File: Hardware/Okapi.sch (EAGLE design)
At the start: 247 parts, among them IC1 ATMEGA1284M, J1 CONN_82.54_SCREW, J3 CONN_42.54_SCREW, J4 CONN_82.54_SCREW, J9 B_SERIES_M.2EKEY_NOPROG, Q1 DMG3404, Q2 DMG3404, Q3 FDN360P, Q4 2N7002, Q5 FDN360P, Q6 DMG3404, Q7 2N7002, Q8 2N7002, U1 TLV61220DBV, U10 TPS22917DBV, U11 SN74AUP1G04YFP, U12 SN74AUP1G04YFP, U13 SN74AUP1G04YFP, U14 SN74AUP2G08DQE, U15 SN74AUP2G08DQE, U16 SN74AUP2G08DQE, U17 MIC2544MSOP, U18 MIC2544MSOP, U19 MIC2544MSOP, U2 TPS62822DLC, U20 MIC2544MSOP, U21 TPS22917DBV, U22 TPS22917DBV, U23 FT231X-Q, U24 SN74LVC1G3157DRL, U25 SN74AUP3G34DCU, U26 TXS0102DQM, U27 TXS0104RGY, U28 TCA9406DCU, U29 TXS0104RGY, U3 TPS61032RSA, U30 MCP4726A2SOT-23, U31 BME280, U32 PAC1934QFN, U33 ADS1115, U34 TXS0102DQM, U35 MB85RC, U36 TCA9406DCU, U37 TLV3691DCK, U38 MLX90393, U39 MIC94094C6, U40 SN74AHC1G86DCK, U41 MCP23018QFN, U42 TXS0104RGY, U43 BMA456, U44 VEML6030, U45 PCA9634QFN, U5 BQ2980RUG, U6 TPS2105, U7 LTC4412S6, U8 TPL5111DDC, U9 TPS79733

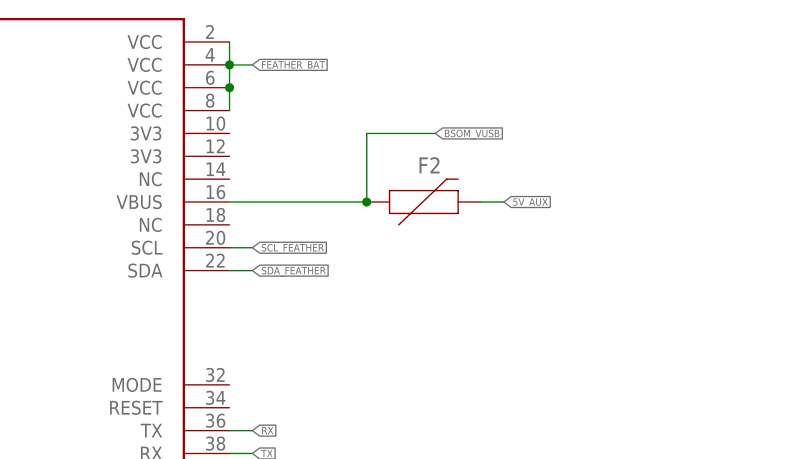
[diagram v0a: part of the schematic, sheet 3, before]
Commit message: Continued design updates
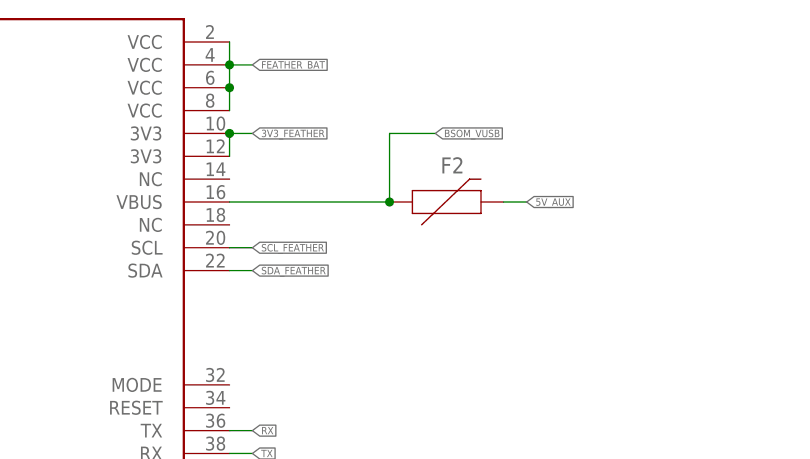
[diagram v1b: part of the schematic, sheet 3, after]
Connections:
- net 3V3_FEATHER: now also J9.3V3@10, J9.3V3@12
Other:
- moved on the sheet: F2
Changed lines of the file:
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@@
 <attribute name="VALUE" x="24.13" y="194.818" size="1.778" layer="96"/>
 </instance>
-<instance part="F2" gate="G$1" x="172.72" y="223.52" smashed="yes">
-<attribute name="NAME" x="174.625" y="226.695" size="1.778" layer="95" font="vector" align="bottom-center"/>
-<attribute name="VALUE" x="173.99" y="220.726" size="1.778" layer="96" font="vector" align="top-center"/>
+<instance part="F2" gate="G$1" x="175.26" y="223.52" smashed="yes">
+<attribute name="NAME" x="177.165" y="226.695" size="1.778" layer="95" font="vector" align="bottom-center"/>
+<attribute name="VALUE" x="176.53" y="220.726" size="1.778" layer="96" font="vector" align="top-center"/>
 </instance>
 <instance part="USB2" gate="G$1" x="68.58" y="228.6" smashed="yes">
@@
 <segment>
 <pinref part="F2" gate="G$1" pin="2"/>
-<wire x1="180.34" y1="223.52" x2="182.88" y2="223.52" width="0.1524" layer="91"/>
-<label x="182.88" y="223.52" size="0.8128" layer="95" xref="yes"/>
+<wire x1="182.88" y1="223.52" x2="185.42" y2="223.52" width="0.1524" layer="91"/>
+<label x="185.42" y="223.52" size="0.8128" layer="95" xref="yes"/>
 </segment>
 </net>
@@
 <label x="2.54" y="205.74" size="0.8128" layer="95" rot="R180" xref="yes"/>
 </segment>
+<segment>
+<pinref part="J9" gate="U1" pin="3V3@10"/>
+<pinref part="J9" gate="U1" pin="3V3@12"/>
+<wire x1="152.4" y1="231.14" x2="152.4" y2="228.6" width="0.1524" layer="91"/>
+<wire x1="152.4" y1="231.14" x2="154.94" y2="231.14" width="0.1524" layer="91"/>
+<junction x="152.4" y="231.14"/>
+<label x="154.94" y="231.14" size="0.8128" layer="95" xref="yes"/>
+</segment>
 </net>
 <net name="SCL_FEATHER" class="0">
@@
 <pinref part="J9" gate="U1" pin="VBUS"/>
 <pinref part="F2" gate="G$1" pin="1"/>
-<wire x1="152.4" y1="223.52" x2="167.64" y2="223.52" width="0.1524" layer="91"/>
-<wire x1="167.64" y1="223.52" x2="167.64" y2="231.14" width="0.1524" layer="91"/>
-<junction x="167.64" y="223.52"/>
-<wire x1="167.64" y1="231.14" x2="175.26" y2="231.14" width="0.1524" layer="91"/>
+<wire x1="152.4" y1="223.52" x2="170.18" y2="223.52" width="0.1524" layer="91"/>
+<wire x1="170.18" y1="223.52" x2="170.18" y2="231.14" width="0.1524" layer="91"/>
+<junction x="170.18" y="223.52"/>
+<wire x1="170.18" y1="231.14" x2="175.26" y2="231.14" width="0.1524" layer="91"/>
 <label x="175.26" y="231.14" size="0.8128" layer="95" xref="yes"/>
 </segment>
